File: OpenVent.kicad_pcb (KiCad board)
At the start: 2 copper layers, 195.5 x 61 mm, 217 parts, among them CN1 2x10_Way_2.54mm_Pitch_Header, J1 OpenVent_Barrel_Connector, Q1 DMMT5401-7-F, Q12 2N7002BK, Q13 2N7002BK, Q14 AOD4185, Q2 AOD4185, Q3 AOD4185, Q4 DMMT5401-7-F, Q5 2N7002BK, Q6 2N7002BK, Q7 2N7002BK, Q8 SSM3K341R, Q9 2N7002BK, U1 TMP236A4DBZT, U10 MPXV4006GP, U11 MPXV4006DP, U12 TLV2333IDR, U13 TLV7042DGKR, U14 LT3796, U15 FT2232HL-REEL, U16 TLV2333IDR, U2 STM32L412R8T6, U3 TI_TXB0108PWR, U4 BD50FC0WEFJ-E2, U5 LDL212D33R, U6 LDL212D33R, U7 LMC6772AIMX, U8 VNH5019ATR-E, U9 LDL212D33R, X1 ABM3B-16.000MHZ, X2 ABM3B-12.000MHZ

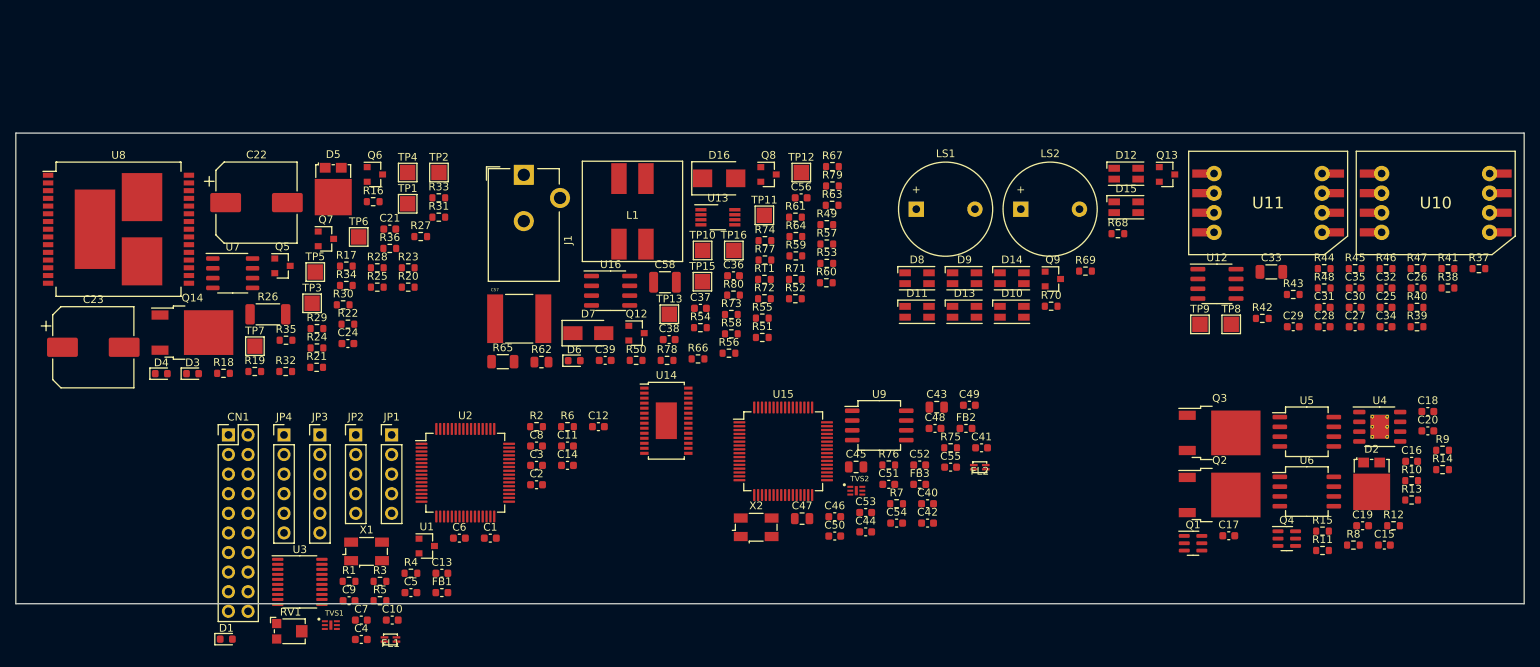
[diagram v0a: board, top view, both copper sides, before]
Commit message: Update OpenVent.kicad_pcb
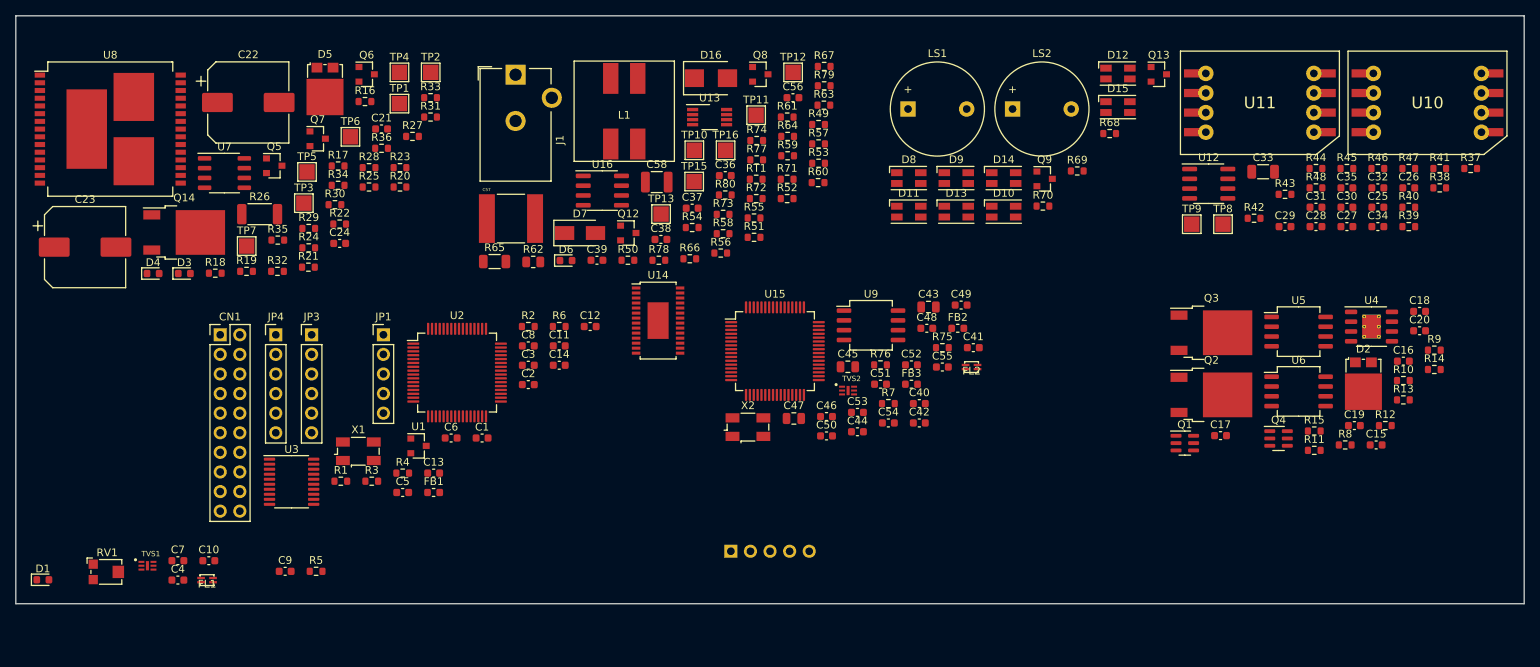
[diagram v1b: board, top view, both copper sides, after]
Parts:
- JP2: moved to B.Cu
- moved JP2 50.9 mm to (142.7, 123.2), turned to 270 degrees
- moved C10 25.0 mm to (75.0, 124.4)
- moved C7 25.0 mm to (71.0, 124.4)
- moved D1 25.0 mm to (53.5, 126.9)
- moved TVS1 25.0 mm to (67.1, 125.1)
- moved C4 25.0 mm to (71.0, 126.9)
- moved FL1 25.0 mm to (74.8, 126.9)
- moved RV1 25.0 mm to (61.8, 125.9)
- moved C15 13.0 mm to (226.3, 109.4)
- moved C16 13.0 mm to (229.8, 98.6)
- moved C40 13.0 mm to (167.1, 104.1)
- moved C41 13.0 mm to (174.1, 96.8)
- moved C53 13.0 mm to (159.1, 105.2)
- moved D3 13.0 mm to (71.8, 87.2)
- moved D4 13.0 mm to (67.8, 87.2)
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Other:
- board size 195.5 x 61 mm -> 195.5 x 76.2 mm
